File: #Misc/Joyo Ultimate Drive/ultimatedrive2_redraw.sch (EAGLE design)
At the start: 33 parts, among them IC1 TL082CP, Q1 2N7000, Q2 2N7000

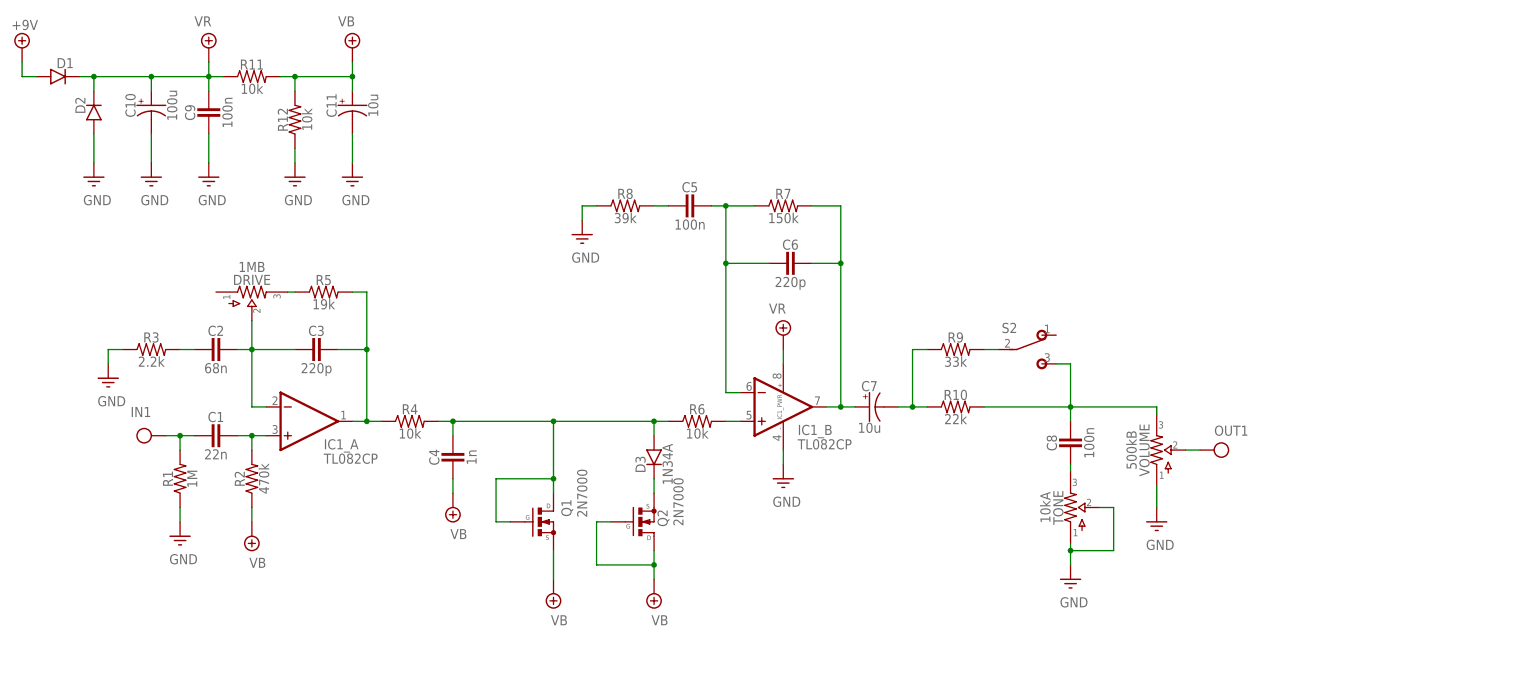
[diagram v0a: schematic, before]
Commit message: 20200322/09:12
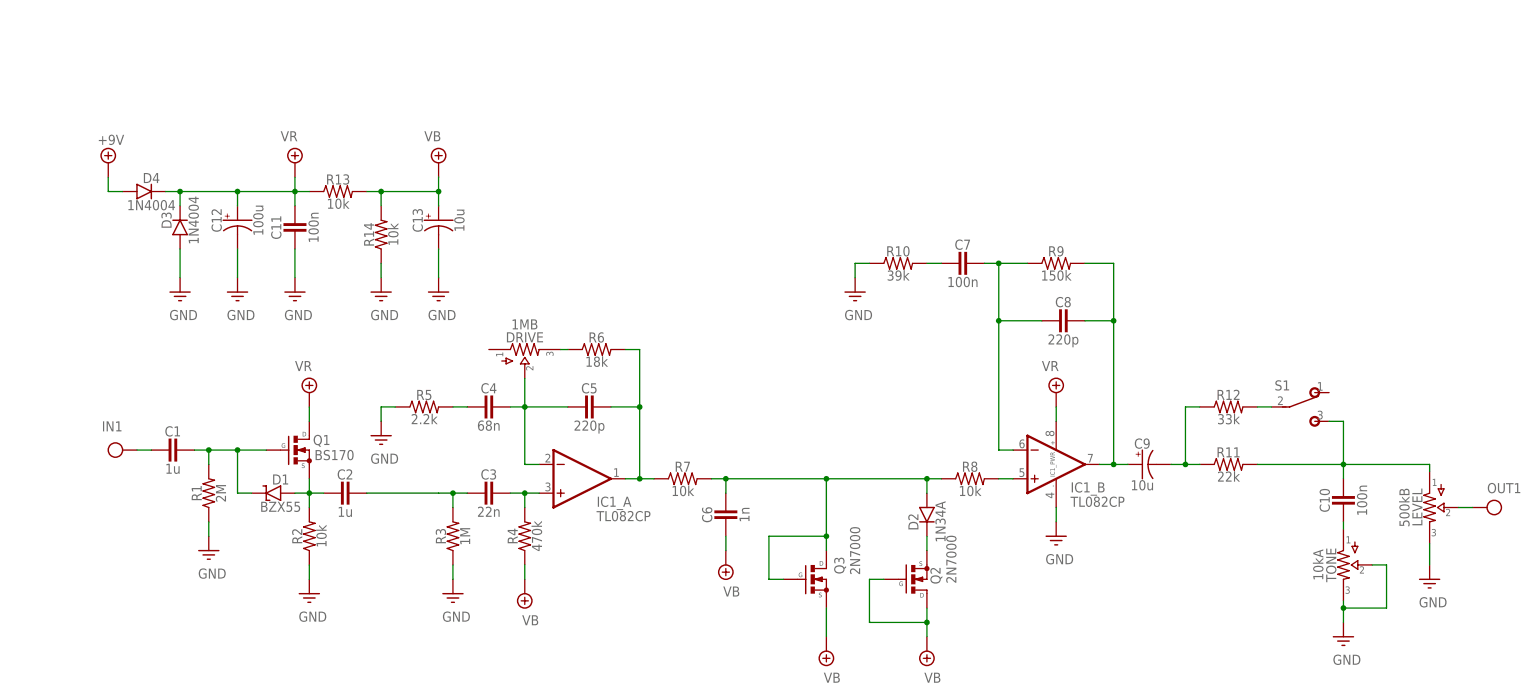
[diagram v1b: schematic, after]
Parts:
- removed S2: (no value), pedals-switches:SPDT
- removed VOLUME: 500kB, pedals-potentiometers:POTS16MM
- added C12: 100u, pedals-capacitors-elec:0500
- added C13: 10u, pedals-capacitors-elec:0500
- added D4: 1N4004, pedals-diodes:DO41.3
- added LEVEL: 500kB, pedals-potentiometers:POTS16MM
- added Q3: 2N7000, pedals-transistors:2N7000
- added R13, R14: 10k, pedals-resistors:R_.3B
- added S1: (no value), pedals-switches:SPDT
- C1: value 22n -> 1u
- C10: value 100u -> 100n; device pedals-capacitors-elec:0500 -> pedals-capacitors-film:CER/FILMBOX.1
- C11, C7: value 10u -> 100n; device pedals-capacitors-elec:0500 -> pedals-capacitors-film:CER/FILMBOX.1
- C2: value 68n -> 1u
- C3: value 220p -> 22n
- C4: value 1n -> 68n
- C5, C8: value 100n -> 220p
- C6: value 220p -> 1n
- C9: value 100n -> 10u; device pedals-capacitors-film:CER/FILMBOX.1 -> pedals-capacitors-elec:0500
- D1: value (none) -> BZX55; device pedals-diodes:DO41.3 -> pedals-diodes:ZENER.3
- D2: value (none) -> 1N34A; device pedals-diodes:DO41.3 -> pedals-diodes:DO41.2
- D3: value 1N34A -> 1N4004; device pedals-diodes:DO41.2 -> pedals-diodes:DO41.3
- Q1: value 2N7000 -> BS170; device pedals-transistors:2N7000 -> pedals-transistors:BS170
- R1: value 1M -> 2M
- R10: value 22k -> 39k
- R11: value 10k -> 22k
- R12: value 10k -> 33k
- R2: value 470k -> 10k
- R3: value 2.2k -> 1M
- R4: value 10k -> 470k
- R5: value 19k -> 2.2k
- R6: value 10k -> 18k
- R7: value 150k -> 10k
- R8: value 39k -> 10k
- R9: value 33k -> 150k
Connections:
- removed net N$17: C8.2, TONE.3
- new net N$2: C10.2, TONE.1
- new net N$21: C1.1, D1.C, Q1.G, R1.2
- new net N$23: C2.2, D1.A, Q1.S, R2.2
- new net N$3: C2.1, C3.2, R3.2
- net +9V: now also D4.A; no longer D1.A
- net GND: now also C11.2, C12.-, C13.-, D3.A, LEVEL.3, R10.1, R14.1, R2.1, R5.1, TONE.3; no longer C10.-, C11.-, C9.2, D2.A, R12.1, R8.1, TONE.1, VOLUME.1
- net IN: no longer R1.2
- net N$1: now also C9.-, R11.1, R12.1; no longer C7.-, R10.1, R9.1
- net N$10: now also D2.C; no longer D3.C
- net N$11: now also C6.1, D2.A, Q3.D, Q3.G, R7.2, R8.1; no longer C4.1, D3.A, Q1.D, Q1.G, R4.2, R6.1
- net N$12: now also C7.1, C8.2, R9.1; no longer C5.1, C6.2, R7.1
- net N$13: now also C8.1, C9.+, R9.2; no longer C6.1, C7.+, R7.2
- net N$14: now also C7.2, R10.2; no longer C5.2, R8.2
- net N$15: now also R12.2, S1.P; no longer R9.2, S2.P
- net N$16: now also C10.1, LEVEL.1, R11.2, S1.S; no longer C8.1, R10.2, S2.S, VOLUME.3
- net N$4: now also C3.1, R4.2; no longer C1.1, R2.2
- net N$5: now also C4.1, C5.2; no longer C2.1, C3.2
- net N$6: now also R6.1; no longer R5.1
- net N$7: now also C5.1, R6.2, R7.1; no longer C3.1, R4.1, R5.2
- net N$8: now also C4.2, R5.2; no longer C2.2, R3.2
- net N$9: now also R8.2; no longer R6.2
- net OUT: now also LEVEL.2; no longer VOLUME.2
- net VB: now also C13.+, C6.2, Q3.S, R13.2, R14.2, R4.1; no longer C11.+, C4.2, Q1.S, R11.2, R12.2, R2.1
- net VR: now also C11.1, C12.+, D3.C, D4.C, Q1.D, R13.1; no longer C10.+, C9.1, D1.C, D2.C, R11.1
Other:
- moved on the sheet: C1, C2, C3, C4, C5, C6, C8, D2, D3, DRIVE, IC1_A, IC1_B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
